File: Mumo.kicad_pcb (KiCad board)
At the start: 2 copper layers, 18 x 13 mm, 20 parts, among them J1 Top_Pins, J2 Bottom Pins, U1 QMC6309, U2 ICM45686, U3 1532H

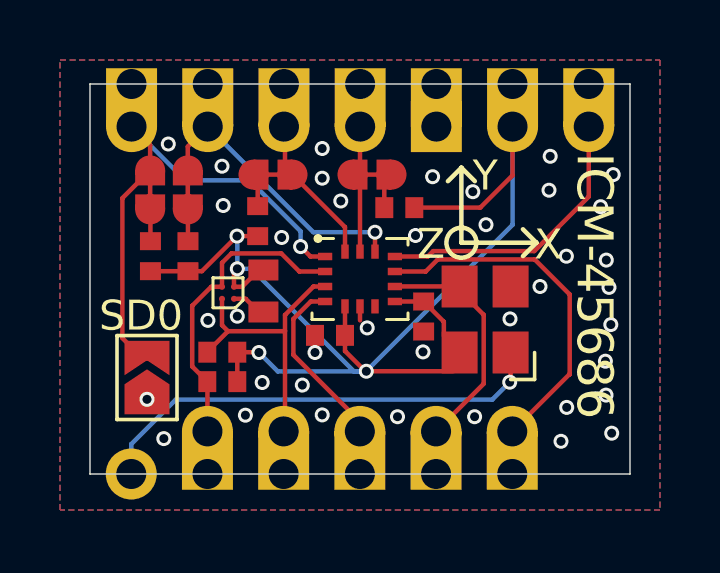
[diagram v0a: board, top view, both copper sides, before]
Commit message: v1.1
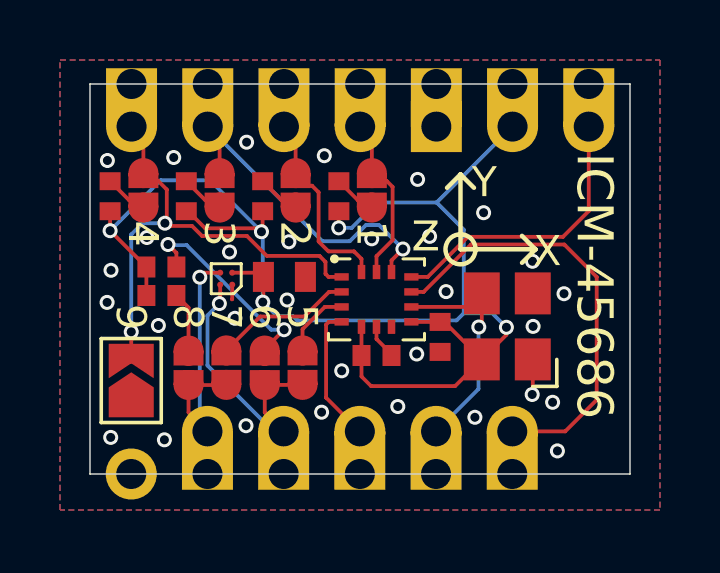
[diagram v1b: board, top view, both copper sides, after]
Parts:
- added G***: LOGO, LOGO, F.Cu at (214.8, 104.3)
- added JP1: SDX_AUX_JMP, Mumo Footprints:JMP_CLSD, F.Cu at (204.5, 110.3)
- added JP2: SCX_PU_JMP, Mumo Footprints:JMP_CLSD, F.Cu at (205.8, 110.3)
- added JP3: SDX_PU_JMP, Mumo Footprints:JMP_CLSD, F.Cu at (203.3, 110.3)
- added JP4: SCX_AUX_JMP, Mumo Footprints:JMP_CLSD, F.Cu at (207.1, 110.3)
- J1: value Top_Pins -> TOP_PINS
- J2: value Bottom Pins -> BOTTOM_PINS
- JP5: renamed from JP1; value JMP -> SCL_PU_JMP
- JP6: renamed from JP2; value JMP -> SDA_PU_JMP
- JP7: renamed from JP3; value JMP -> CS_PU_JMP
- JP8: renamed from JP4; value JMP -> SD0_PU_JMP
- JP9: renamed from JP5; value SD0_JMP -> SD0_GND_JMP
- moved C2 3.67 mm to (211.7, 109.2), turned to 90 degrees
- moved R2 3.52 mm to (202.4, 107.8), turned to 0 degrees
- moved R1 3.49 mm to (202.4, 106.9), turned to 0 degrees
- moved R6 2.41 mm to (200.7, 104.5)
- moved R3 2.05 mm to (208.3, 104.5), turned to 90 degrees
- moved C1 2.04 mm to (209.6, 109.8), turned to 0 degrees
- moved R5 2.00 mm to (203.2, 104.5)
- moved JP7 1.06 mm to (204.3, 104.3)
- moved JP6 0.92 mm to (206.9, 104.3), turned to -90 degrees
- moved U2 0.87 mm to (209.6, 108.0)
- moved R4 0.85 mm to (205.8, 104.5)
- moved C3 0.84 mm to (206.5, 107.2), turned to 0 degrees
- moved U3 0.77 mm to (213.9, 108.9)
- moved JP9 0.53 mm to (201.4, 110.7)
- moved JP5 0.53 mm to (209.4, 104.3), turned to -90 degrees
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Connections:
- net CLK renamed /CLK
- net CLK_CTL renamed /CLK_CTL
- net CS renamed /CS
- net INT1 renamed /INT1
- net OCS renamed /OCS
- net OSDO renamed /OSDO
- net SCL renamed /SCL
- net SD0 renamed /SD0
- net SDA renamed /SDA
- J2 pad 4: SCX -> /SCX
- J2 pad 5: SDX -> /SDX
- R1 pad 2: SCX -> Net-(JP2-B)
- R2 pad 2: SDX -> Net-(JP3-B)
- U1 pad A2: SCX -> /SCX
- U1 pad B2: SDX -> /SDX
- U2 pad 2: SDX -> Net-(JP1-A)
- U2 pad 3: SCX -> Net-(JP4-A)
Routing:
- net SDX: track 10.3 -> 0.00 mm
- net SCX: track 9.68 -> 0.00 mm
- net /SCX: track 0.00 -> 9.39 mm, vias 0 -> 1
- net /SDX: track 0.00 -> 9.06 mm, vias 0 -> 1
- net Net-(JP2-B): track 0.00 -> 6.87 mm, vias 0 -> 2
- net +3V3: track 42.1 -> 48.5 mm, vias 4 -> 5
- net Net-(JP1-A): track 0.00 -> 4.65 mm
- net /OCS: track 11.8 -> 14.6 mm
- net Net-(JP4-A): track 0.00 -> 2.32 mm
- net Net-(JP3-B): track 0.00 -> 2.00 mm
- net /CS: track 9.42 -> 11.3 mm
- net /SDA: track 4.91 -> 6.39 mm
- net /INT1: track 5.97 -> 4.58 mm
- net /SCL: track 4.17 -> 5.55 mm
- net /CLK_CTL: track 15.2 -> 16.5 mm
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- added copper zone on In1.Cu, net GND
- added copper zone on In2.Cu, net GND
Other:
- copper layers 2 -> 4
- board text added: "1"
- board text added: "2"
- board text added: "3"
- board text added: "4"
- board text added: "5"
- board text added: "6"
- board text added: "7"
- board text added: "8"
- board text added: "9"
